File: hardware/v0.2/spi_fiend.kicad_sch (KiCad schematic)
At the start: 25 parts, among them J1 USB_C_Receptacle_USB2.0, J2 CONN_01X04, J3 CONN_01X07, J4 PROG HEADER, J5 CONN_01X05, SW1 switch_no, SW2 switch_no, U1 STM32F042G6U6, U2 DRTR5V0U4S, U3 XC6222B331MR-G

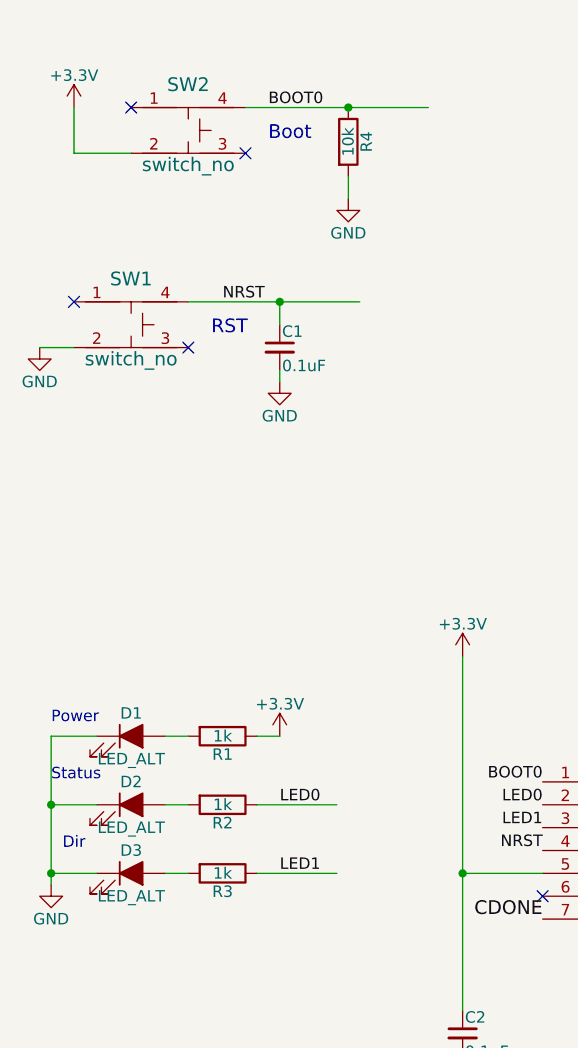
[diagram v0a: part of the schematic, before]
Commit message: P&R almost done.
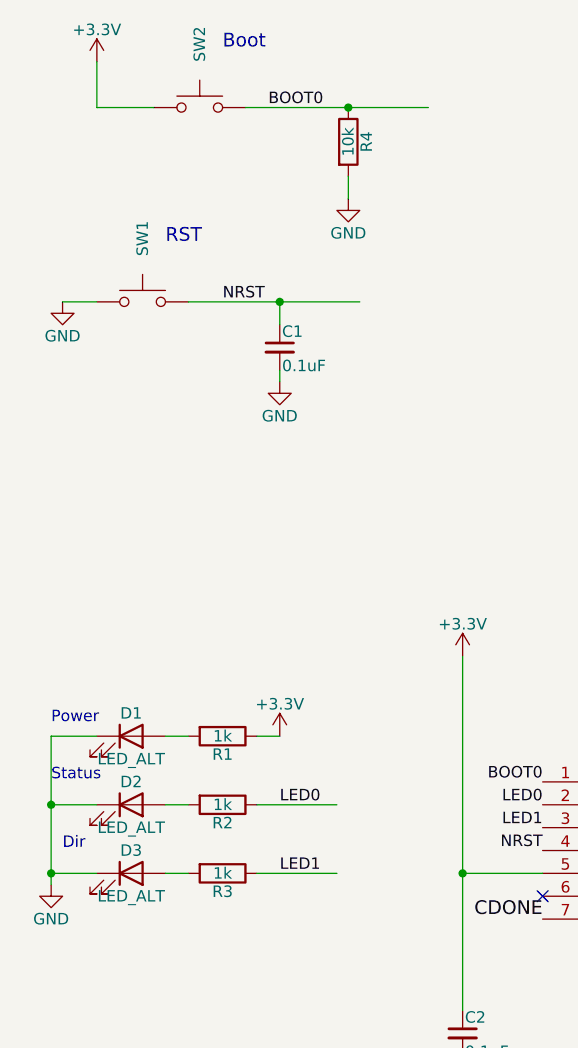
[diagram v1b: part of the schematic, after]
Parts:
- removed SW1: switch_no, footprints:PUSHBUTTON_SMD_KMR2, symbol spi_fiend-rescue:switch_no-emeb_library
- removed SW2: switch_no, Button_Switch_SMD:SW_Push_1P1T_NO_CK_KMR2, symbol spi_fiend-rescue:switch_no-emeb_library
- added SW1, SW2: SW_Push, emeb_library:SW_SPST_PTS815, symbol Switch:SW_Push
- D1, D2, D3: symbol spi_fiend-rescue:LED_ALT-Device -> Device:LED
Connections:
- net +3V3 is gone; now on net +3.3V: C2.1, C3.1, J5.1 (Pin_1), R1.1, U1.17 (VDD), U1.18 (VDDIO2), U1.5 (VDDA)
- net +3.3V: now also SW2.1
- net BOOT0: now also SW2.2
- net GND: now also SW1.1
- net NRST: now also SW1.2
- no-connect marks 14 -> 10

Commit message: Revert "P&R almost done."
This reverts commit 97a49ac74aeb3e6297260b20c9d5898586bb1314.
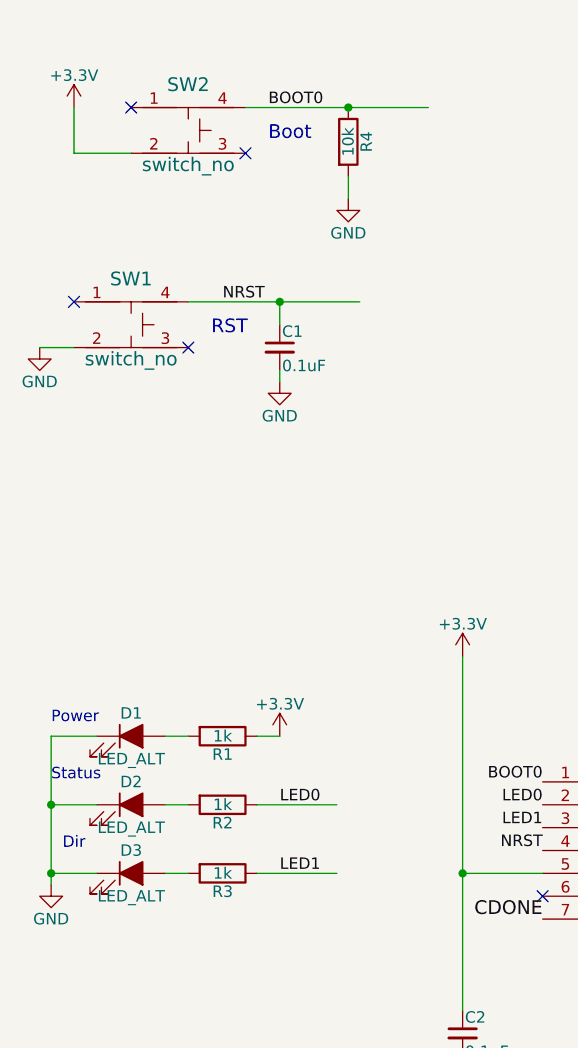
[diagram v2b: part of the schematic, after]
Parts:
- removed SW1, SW2: SW_Push, emeb_library:SW_SPST_PTS815, symbol Switch:SW_Push
- added SW1: switch_no, footprints:PUSHBUTTON_SMD_KMR2, symbol spi_fiend-rescue:switch_no-emeb_library
- added SW2: switch_no, Button_Switch_SMD:SW_Push_1P1T_NO_CK_KMR2, symbol spi_fiend-rescue:switch_no-emeb_library
- D1, D2, D3: symbol Device:LED -> spi_fiend-rescue:LED_ALT-Device
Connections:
- net +3.3V: no longer C2.1, C3.1, J5.1 (Pin_1), R1.1, U1.17 (VDD), U1.18 (VDDIO2), U1.5 (VDDA)
- net BOOT0: now also SW2.4
- net GND: now also SW1.2
- net NRST: now also SW1.4
- new net +3V3: C2.1, C3.1, J5.1 (Pin_1), R1.1, SW2.2, U1.17 (VDD), U1.18 (VDDIO2), U1.5 (VDDA)
- no-connect marks 10 -> 14
